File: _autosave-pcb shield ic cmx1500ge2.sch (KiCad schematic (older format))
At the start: 52 parts, among them J1 SMA, J2 U.FL, J3 Conn_01x01_Male, J4 Conn_01x01_Male, P1 Power, P2 Analog, P3 Digital, P4 Digital, P5 HEADER2x4, P6 HEADER-1X6, P7 Communication, Q1 BSS138, Q2 BSS138, Q3 BSS138, U1 CXM1500GE, U2 TXS0108EPW, U3 LM1117-Adj, U4 ADS1115

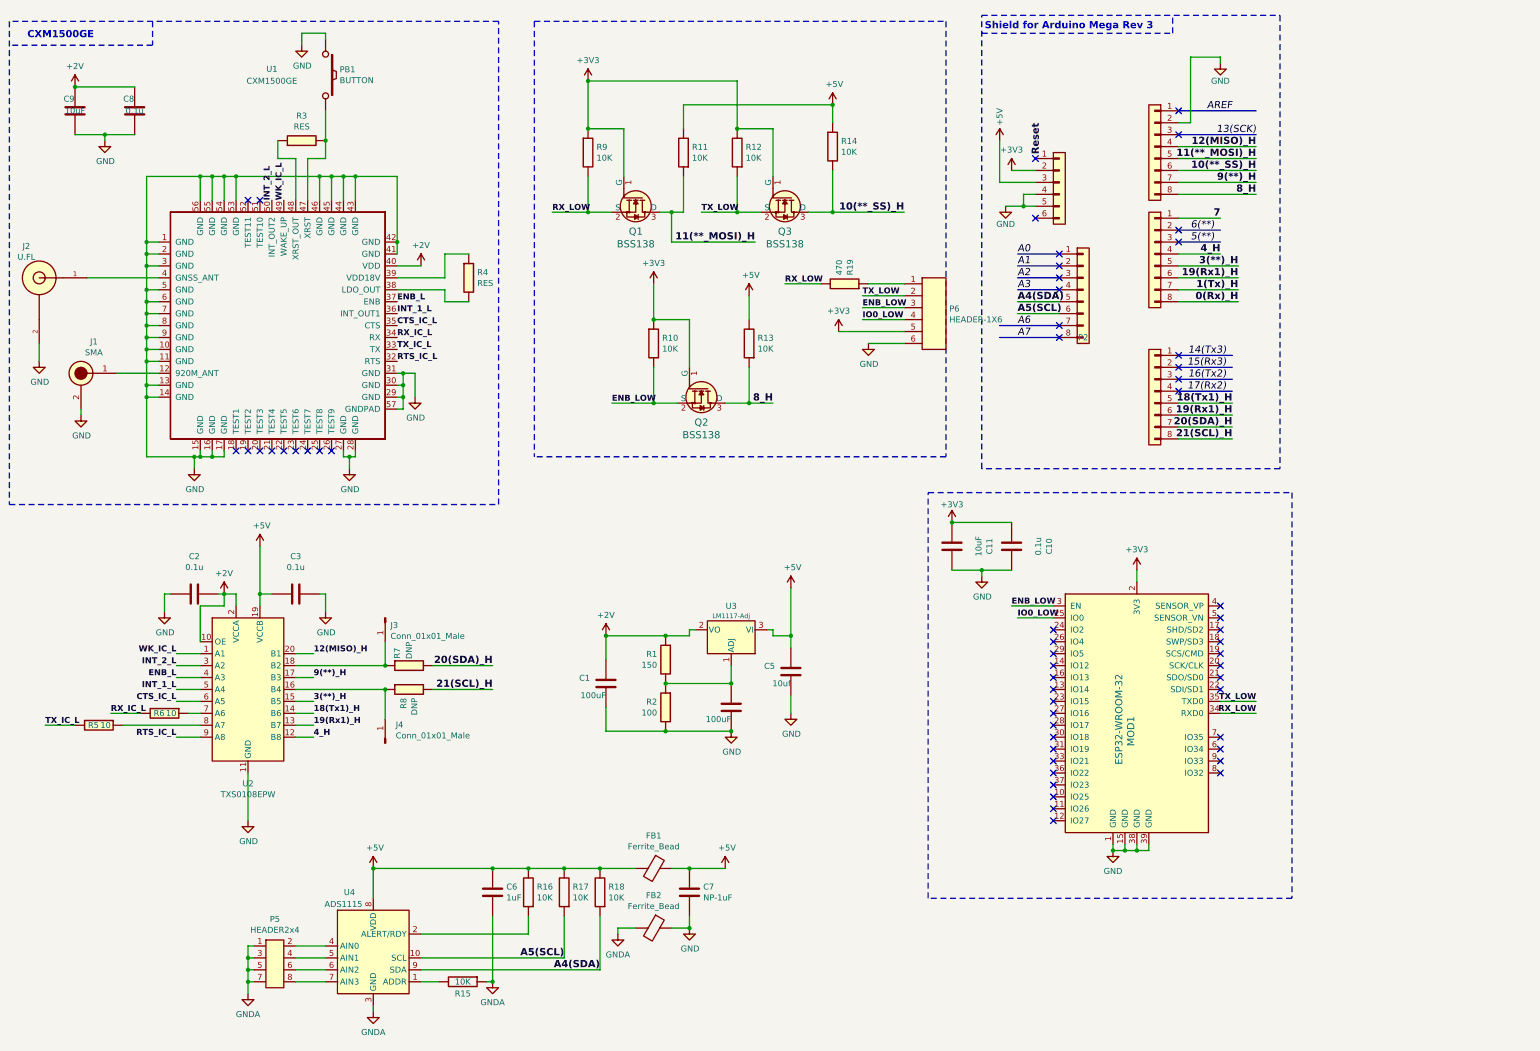
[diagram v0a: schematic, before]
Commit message: initial Commit
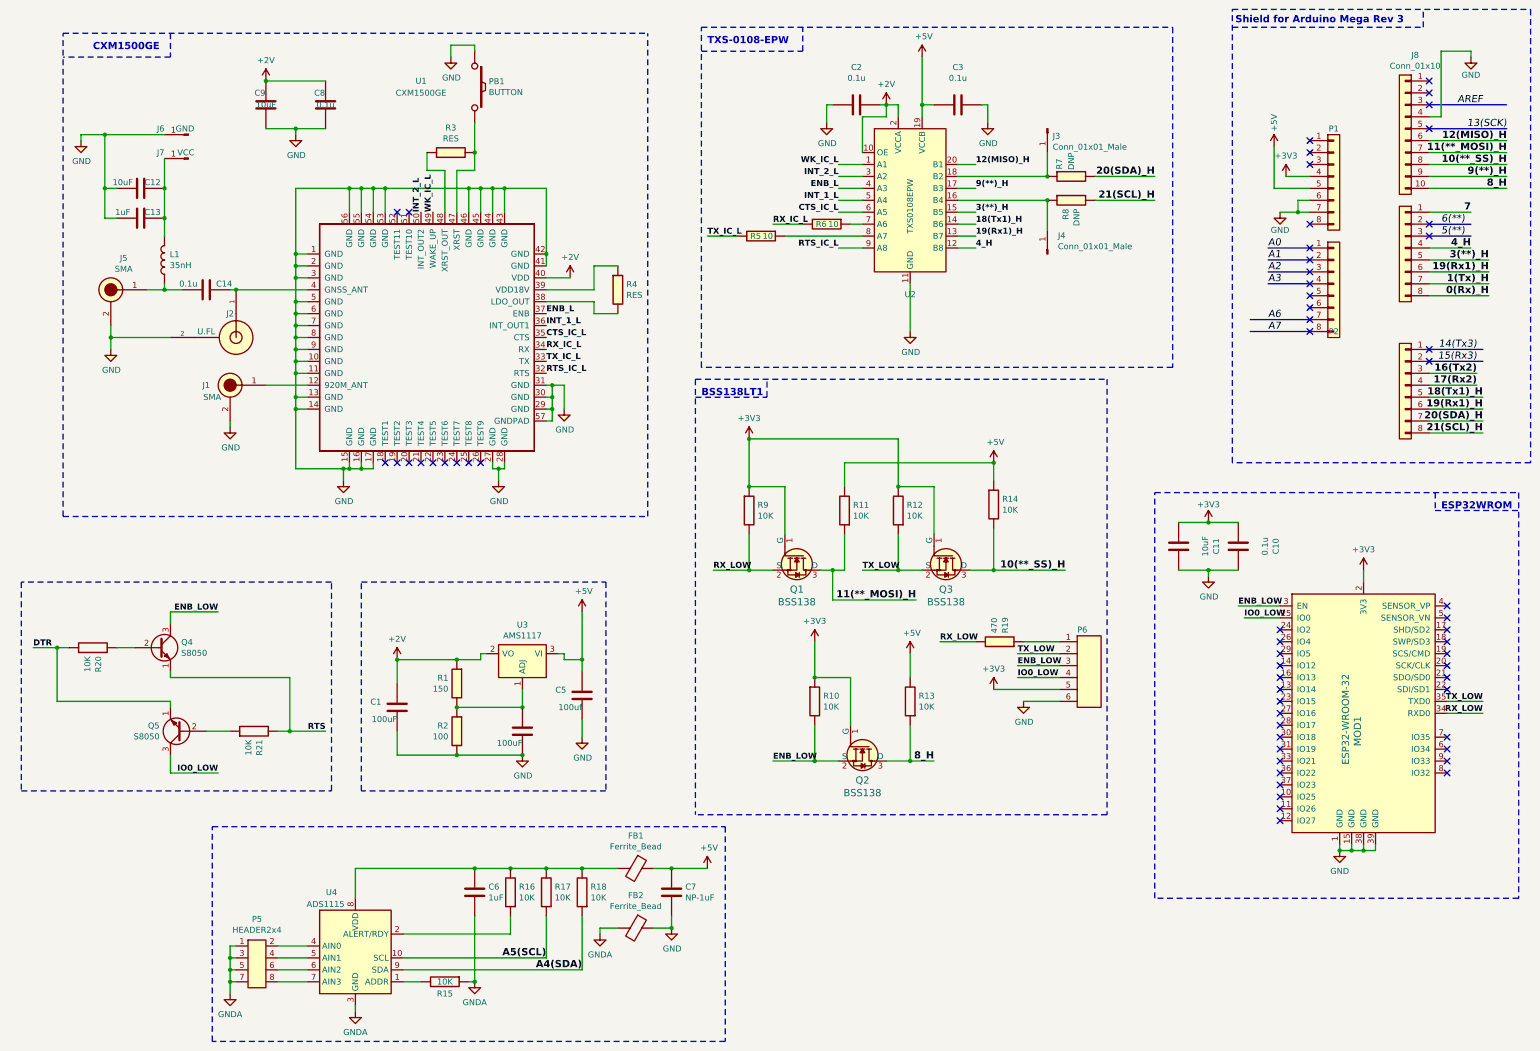
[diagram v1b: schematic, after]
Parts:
- removed P1: Power, Socket_Arduino_Uno:Socket_Strip_Arduino_1x06, symbol Connector_Generic:Conn_01x06
- removed P3: Digital, Socket_Arduino_Uno:Socket_Strip_Arduino_1x08, symbol Connector_Generic:Conn_01x08
- removed U3: LM1117-Adj, smd:TO261AA-LM1117_rev, symbol Regulator_Linear:LM1117-ADJ
- added C12: 10uF, Capasitor:C_Ceramic_SMD_0603, symbol Capacitor:NP-10nF
- added C13: 1uF, Capasitor:C_Ceramic_SMD_0603, symbol Capacitor:NP-10nF
- added C14: 0.1u, Capasitor:C_Ceramic_SMD_0603, symbol Capacitor:NP-10nF
- added J5: SMA, Connectors_SMA:SMA_Male_Angled_TH, symbol Miscellaneous_Connectors:SMA
- added J6: GND, Headers:Pin_Header_1x01_Male_10mil_Straight_TH, symbol Connector:Conn_01x01_Male
- added J7: VCC, Headers:Pin_Header_1x01_Male_10mil_Straight_TH, symbol Connector:Conn_01x01_Male
- added J8: Conn_01x10, Connector_PinHeader_2.54mm:PinHeader_1x10_P2.54mm_Vertical, symbol Connector_Generic:Conn_01x10
- added L1: 35nH, Inductor:L_0805_2012Metric, symbol Inductor:10uH_0.5A
- added P1: Analog, Socket_Arduino_Uno:Socket_Strip_Arduino_1x08, symbol Connector_Generic:Conn_01x08
- added Q4, Q5: S8050, digikey-footprints:SOT-23-3, symbol Transistor_BJT:S8050
- added R20, R21: 10K, resistor:R_Chip_SMD_0603, symbol Resistor:10K_0.100W
- added U3: AMS1117, Package_TO_SOT_SMD:SOT-223-3_TabPin2, symbol Regulator_Linear:AMS1117
- C10, C3, C8: Manf# (none) -> 399-5784-2-ND
- C2: manf# (none) -> 399-5784-2-ND
- C5: value 10uf -> 100uf
- P5: footprint Connector_PinHeader_2.00mm:PinHeader_2x04_P2.00mm_Vertical -> Connector_PinHeader_2.54mm:PinHeader_2x04_P2.54mm_Vertical
- P6: footprint Connector_PinHeader_2.00mm:PinHeader_1x06_P2.00mm_Vertical -> Connector_PinHeader_2.54mm:PinHeader_1x06_P2.54mm_Vertical
- U2: Manufacturer (none) -> Texas Instruments; manf# (none) -> TXS0108EPWR; part# (none) -> 296-23011-2-ND
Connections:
- net +2V5: now also U3.2 (VO)
- net +3V3: now also P1.4 (Pin_4)
- net +5V: now also P1.5 (Pin_5), U3.3 (VI); no longer C6.2, FB1.2, R16.2, R17.2, R18.2, U4.8 (VDD)
- net 10(**_SS)_H: now also J8.8 (Pin_8)
- net 11(**_MOSI)_H: now also J8.7 (Pin_7)
- net 12(MISO)_H: now also J8.6 (Pin_6)
- net 16(Tx2): now also P7.3 (Pin_3)
- net 17(Rx2): now also P7.4 (Pin_4)
- net 8_H: now also J8.10 (Pin_10)
- net 9(**)_H: now also J8.9 (Pin_9)
- net A4(SDA): no longer P2.5 (Pin_5)
- net A5(SCL): no longer P2.6 (Pin_6)
- net ENB_LOW: now also Q4.3 (C)
- net GND: now also C12.2, C13.2, J5.2 (GND), J6.1 (Pin_1), J8.4 (Pin_4), P1.6 (Pin_6), P1.7 (Pin_7)
- net IO0_LOW: now also Q5.3 (C)
- net at J2.1, U1.4 (GNSS_ANT): now also C14.1
- net at C4.1, R1.2, R2.1: now also U3.1 (ADJ)
- new net: Q4.2 (B), R20.2
- new net: Q5.2 (B), R21.1
- new net: C14.2, J5.1 (RF), L1.1
- new net: C12.1, C13.1, J7.1 (Pin_1), L1.2
- new net: C6.2, FB1.2, R16.2, R17.2, R18.2, U4.8 (VDD)
- new net DTR: Q5.1 (E), R20.1
- new net RTS: Q4.1 (E), R21.2
- no-connect marks 56 -> 60
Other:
- note added: "BSS138LT1\n"
- note added: "ESP32WROM\n"
- note added: "TXS-0108-EPW\n"
- moved on the sheet: C1, C10, C11, C2, C3, C5, C6, C7, C8, C9, FB1, FB2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
